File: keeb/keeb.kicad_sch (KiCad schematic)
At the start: 161 parts, among them J101 AVR-ISP-6, J102 USB_C_Receptacle_USB2.0, SW101 SW_Push, SW102 SW_Push, SW103 SW_Push, SW104 SW_Push, SW105 SW_Push, SW106 SW_Push, SW107 SW_Push, SW108 SW_Push, SW109 SW_Push, SW110 SW_Push, SW111 SW_Push, SW112 SW_Push, SW113 SW_Push, SW114 SW_Push, SW115 SW_Push, SW116 SW_Push, SW117 SW_Push, SW118 SW_Push, SW119 SW_Push, SW120 SW_Push, SW121 SW_Push, SW122 SW_Push, SW123 SW_Push, SW124 SW_Push, SW125 SW_Push, SW126 SW_Push, SW127 SW_Push, SW128 SW_Push, SW129 SW_Push, SW130 SW_Push, SW131 SW_Push, SW132 SW_Push, SW133 SW_Push, SW134 SW_Push, SW135 SW_Push, SW136 SW_Push, SW137 SW_Push, SW138 SW_Push, SW139 SW_Push, SW140 SW_Push, SW141 SW_Push, SW142 SW_Push, SW143 SW_Push, SW144 SW_Push, SW145 SW_Push, SW146 SW_Push, SW147 SW_Push, SW148 SW_Push, SW149 SW_Push, SW150 SW_Push, SW151 SW_Push, SW152 SW_Push, SW153 SW_Push, SW154 SW_Push, SW155 SW_Push, SW156 SW_Push, SW157 SW_Push, SW158 SW_Push, SW159 SW_Push, SW160 SW_Push, SW161 SW_Push, SW162 SW_Push, SW163 SW_Push, SW164 SW_Push, SW165 SW_Push, SW166 SW_Push, SW167 SW_Push, U101 ATmega32U4-AU, Y101 16Mhz

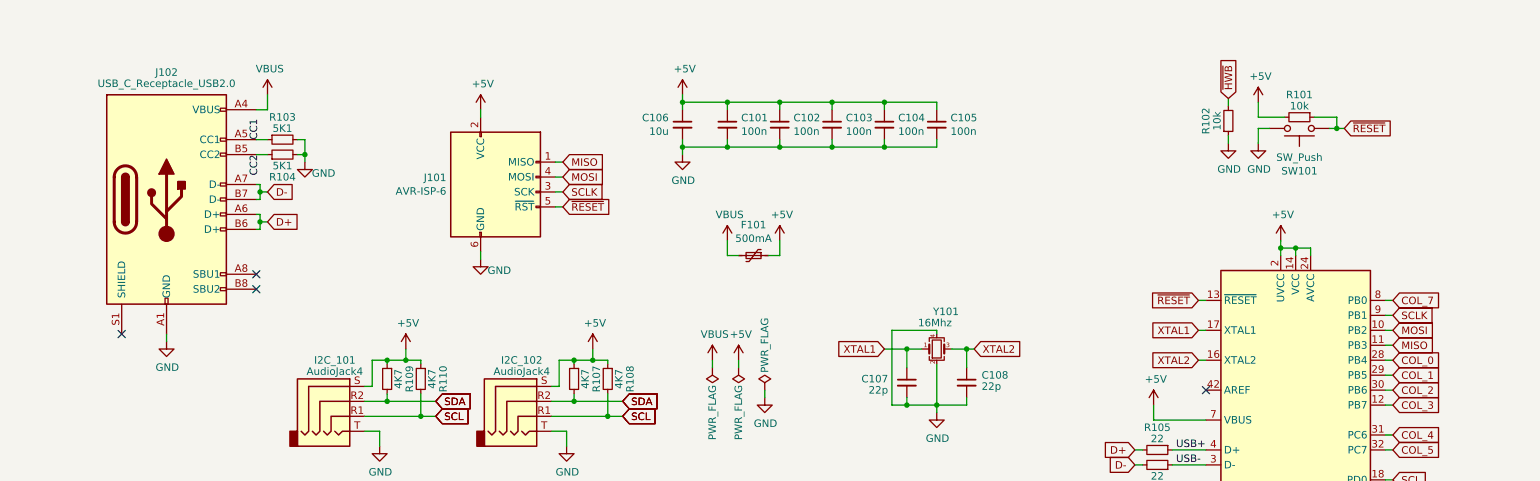
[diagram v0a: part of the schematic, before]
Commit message: RESTART: Version2
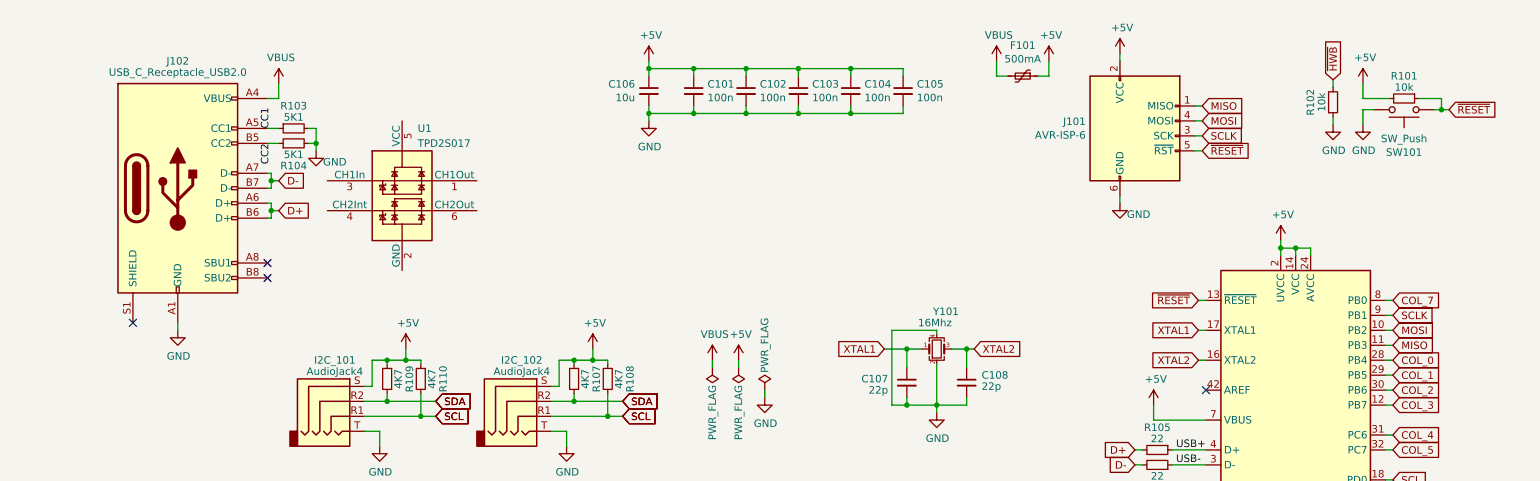
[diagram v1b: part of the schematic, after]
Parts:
- added U1: TPD2S017, Package_TO_SOT_SMD:SOT-23-6, symbol Power_Protection:TPD2S017
- I2C_101, I2C_102: footprint unORTHOdox_CF:Jack_3.5mm_TIC54-00177_Horizontal -> unORTHOdox:Jack_3.5mm_TIC54-00177_Horizontal
- J101: footprint Connector_PinHeader_2.54mm:PinHeader_2x03_P2.54mm_Vertical -> Stamp_Attach:Stamp-Attach_SA2030-IDC-NL_2x03_P1.27mm_Vertical
- J102: footprint unORTHOdox_CF:USB_C_Receptacle_HRO_TYPE-C-31-M-12 -> unORTHOdox:USB_C_Receptacle_HRO_TYPE-C-31-M-12
- SW102: footprint Switch_Keyboard_Cherry_MX:SW_Cherry_MX_PCB_1.00u -> PCM_Switch_Keyboard_Cherry_MX:SW_Cherry_MX_PCB_1.00u
- U101: footprint Package_DFN_QFN:QFN-44-1EP_7x7mm_P0.5mm_EP5.2x5.2mm -> unORTHOdox:QFN-44-1EP_7x7mm_P0.5mm_EP5.2x5.2mm
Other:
- moved on the sheet: C101, C102, C103, C104, C105, C106, F101, J101, J102, R101, R102, R103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
